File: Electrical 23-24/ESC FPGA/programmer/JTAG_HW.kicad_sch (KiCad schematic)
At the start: 44 parts, among them J1 USB_B_Micro, J2 SFH11-PBPC-D07-ST-BK, J3 Conn_01x05_Pin, J4 Conn_01x11_Pin, J5 Conn_01x14_Pin, SW1 SW_DPST, U1 93CxxC, U2 AMS1117-3.3, U3 NUP2202, U4 FT2232HL, Y1 12MHZ

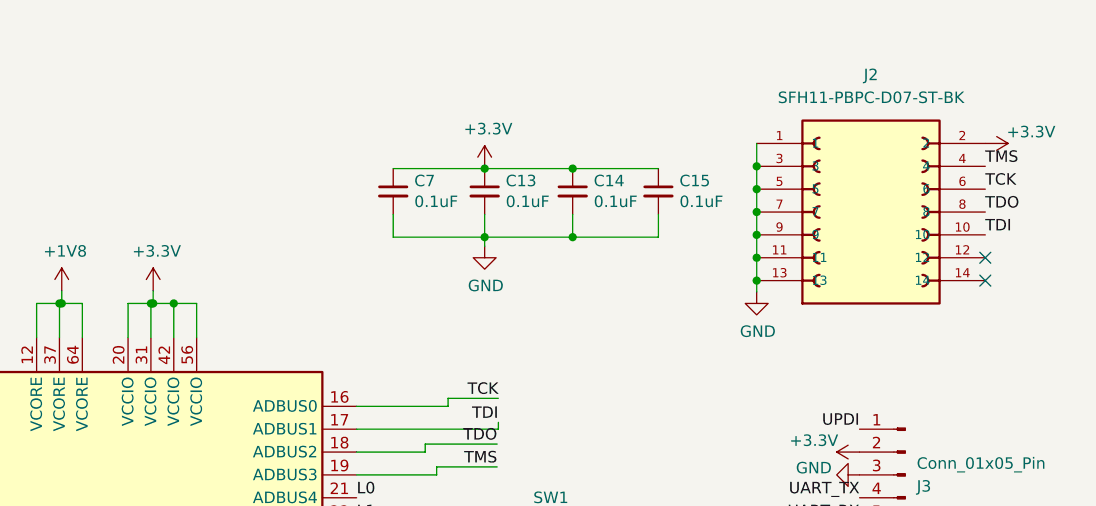
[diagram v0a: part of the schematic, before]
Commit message: idk but something
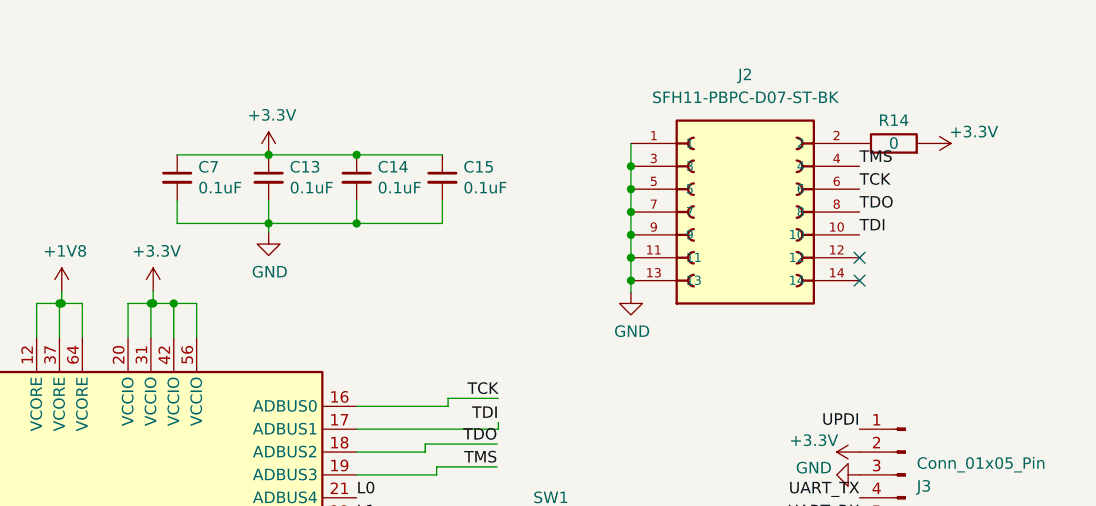
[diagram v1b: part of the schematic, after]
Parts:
- added R14: 0, symbol Device:R
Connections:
- net +3.3V: now also R14.2; no longer J2.2
- new net: J2.2, R14.1
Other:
- moved on the sheet: C13, C14, C15, C7, J2
